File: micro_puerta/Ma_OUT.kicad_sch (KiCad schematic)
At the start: 6 parts

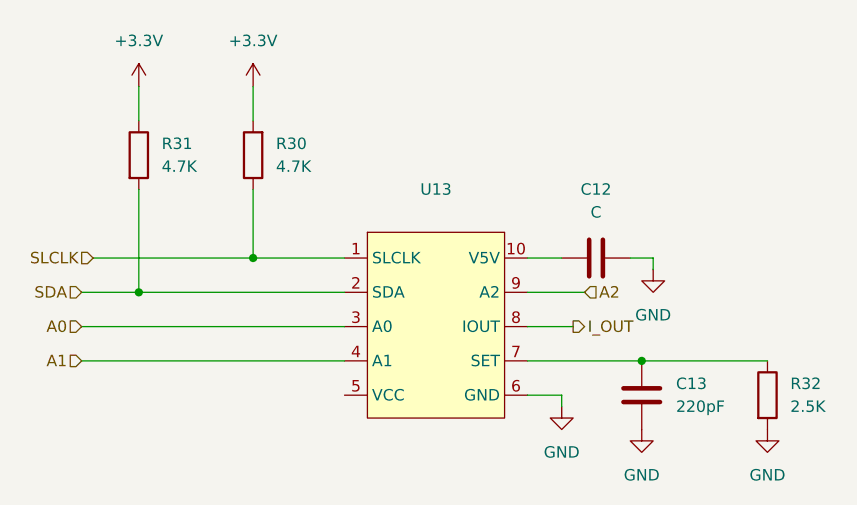
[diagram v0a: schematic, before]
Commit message: actualizacion placa
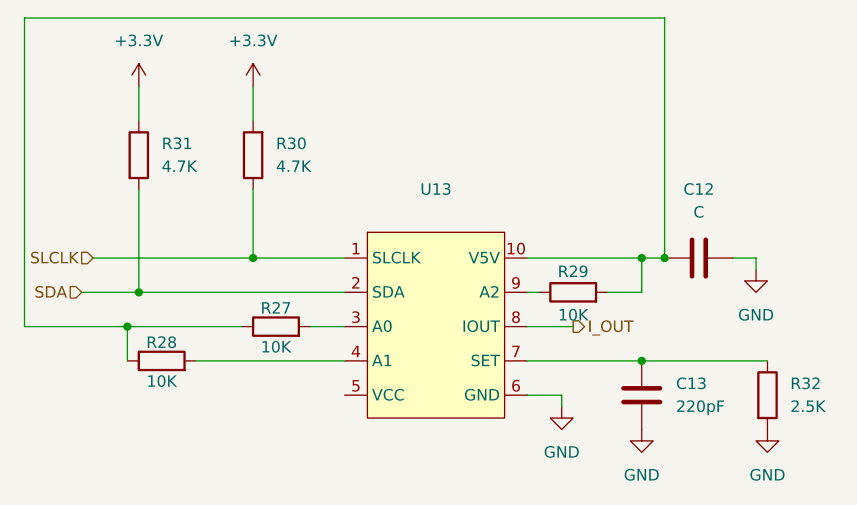
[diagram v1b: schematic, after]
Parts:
- added R27, R28, R29: 10K, symbol Device:R
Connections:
- net at C12.1, U13.10 (V5V): now also R27.1, R28.1, R29.2
- net A0: no longer names the net of U13.3 (A0)
- net A0: now also R27.2
- net A1: no longer names the net of U13.4 (A1)
- net A1: now also R28.2
- net A2: no longer names the net of U13.9 (A2)
- net A2: now also R29.1
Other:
- moved on the sheet: C12
